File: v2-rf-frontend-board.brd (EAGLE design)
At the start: 86.6 x 43.9 mm, 150 parts, among them J1 1.27MM-SWD-CONNECTOR, J2 CON_SMA-ENDFIRE_EMERSON_EMERS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, J3 ROCKETNET-CONNECTOR-16M, J4 ZX62D-B-5P8, J5 BREAKOUT, J7 CON_HIROSE_DM3D(MICROSD), Q1 NTR4101P, T1 ALT4532, T2 ALT4532, U1 MAX2769, U2 STM32F4V_100PIN_GPSBOARD, U3 KSZ8081, U4 7Q-16.368MBG-T, U5 XC2401A8167R-G, U6 MAX8510EXK29+T, U7 MAX8510EXK29+T, U8 LMZ12001, X1 25 MHz

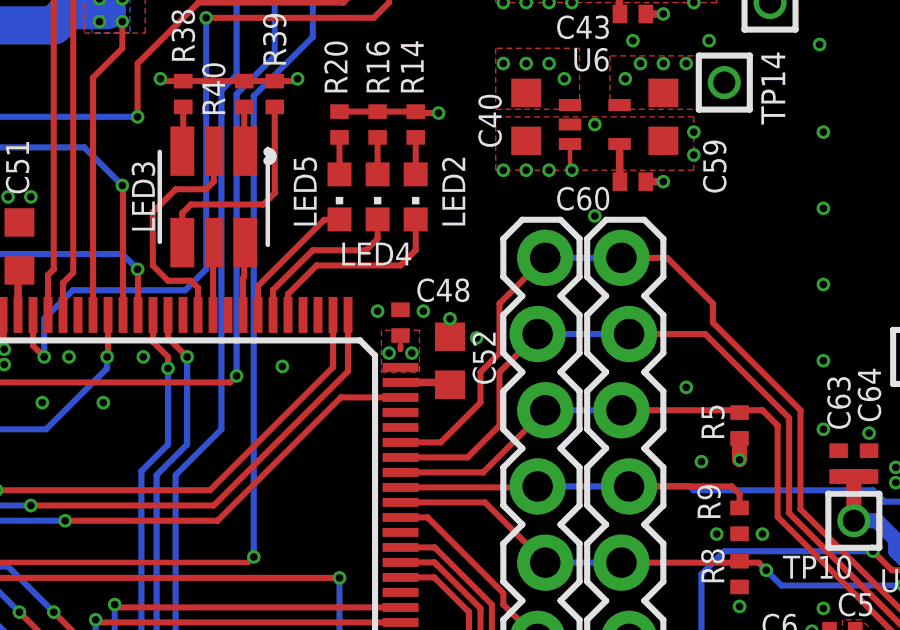
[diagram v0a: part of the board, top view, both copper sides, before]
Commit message: Silly clean up, ran ERC and DRC again.
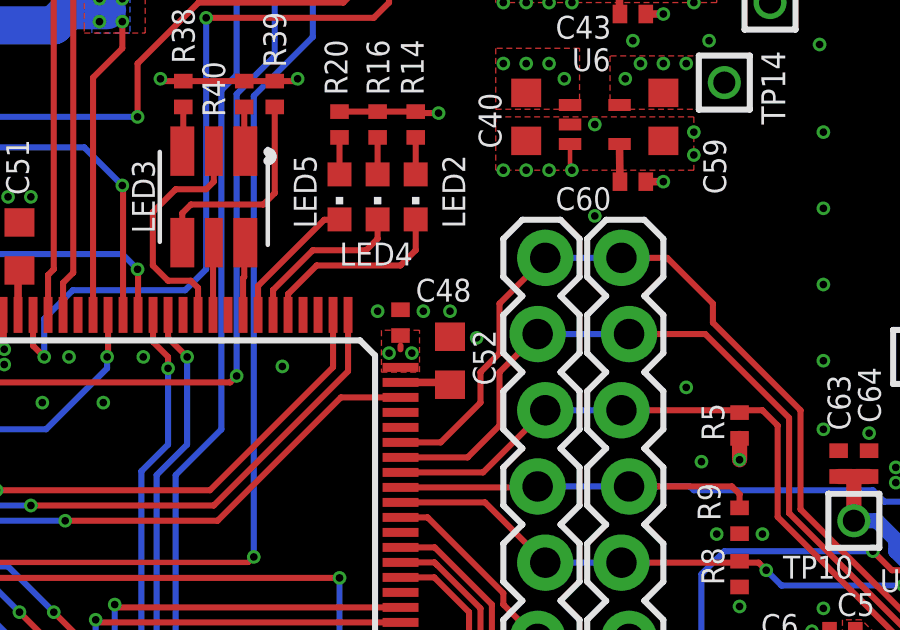
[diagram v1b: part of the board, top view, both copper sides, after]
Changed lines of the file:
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@@
 <layer number="23" name="tOrigins" color="15" fill="1" visible="yes" active="yes"/>
 <layer number="24" name="bOrigins" color="15" fill="1" visible="yes" active="yes"/>
-<layer number="25" name="tNames" color="7" fill="1" visible="yes" active="yes"/>
+<layer number="25" name="tNames" color="7" fill="1" visible="no" active="yes"/>
 <layer number="26" name="bNames" color="7" fill="1" visible="no" active="yes"/>
 <layer number="27" name="tValues" color="7" fill="1" visible="no" active="yes"/>
@@
 <via x="28.067" y="36.83" extent="1-16" drill="0.254"/>
 <via x="40.64" y="38.227" extent="1-16" drill="0.254"/>
-<via x="58.674" y="26.797" extent="1-16" drill="0.254"/>
+<via x="58.674" y="27.051" extent="1-16" drill="0.254"/>
 <via x="74.93" y="41.91" extent="1-16" drill="0.254"/>
 <via x="76.581" y="21.463" extent="1-16" drill="0.254"/>

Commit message: Added modwire proposals for SPI 3-wire fix. See Issue 4 in gps-rf-board github repository.
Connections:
- net MAX_CFG_!CS: now also U2.96
- net MAX_CFG_MOSI: now also U2.54
- net MAX_CFG_SCLK: now also U2.47
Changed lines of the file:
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@@
 <wire x1="69.977" y1="20.32" x2="69.977" y2="23.495" width="0.2032" layer="1"/>
 <wire x1="69.977" y1="23.495" x2="67.183" y2="26.289" width="0.2032" layer="1"/>
+<contactref element="U2" pad="47"/>
+<wire x1="57.026" y1="22.177" x2="57.026" y2="23.677" width="0" layer="19" extent="1-1"/>
 </signal>
 <signal name="MAX_CFG_MOSI">
@@
 <wire x1="70.358" y1="20.447" x2="70.358" y2="23.749" width="0.2032" layer="1"/>
 <wire x1="70.358" y1="23.749" x2="67.437" y2="26.67" width="0.2032" layer="1"/>
+<contactref element="U2" pad="54"/>
+<wire x1="57.026" y1="22.677" x2="53.776" y2="26.927" width="0" layer="19" extent="1-1"/>
 </signal>
 <signal name="MAX_CFG_!CS">
@@
 <wire x1="57.026" y1="21.677" x2="59.777" y2="21.677" width="0.2032" layer="1"/>
 <wire x1="59.777" y1="21.677" x2="61.849" y2="23.749" width="0.2032" layer="1"/>
+<contactref element="U2" pad="96"/>
+<wire x1="41.526" y1="15.177" x2="57.026" y2="21.677" width="0" layer="19" extent="1-1"/>
 </signal>
 <signal name="N$9">

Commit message: Removed SPI2_NSS modwire proposal from v2 schematic.
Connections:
- net MAX_CFG_!CS: no longer U2.96
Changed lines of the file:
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@@
 <wire x1="57.026" y1="21.677" x2="59.777" y2="21.677" width="0.2032" layer="1"/>
 <wire x1="59.777" y1="21.677" x2="61.849" y2="23.749" width="0.2032" layer="1"/>
-<contactref element="U2" pad="96"/>
-<wire x1="41.526" y1="15.177" x2="57.026" y2="21.677" width="0" layer="19" extent="1-1"/>
 </signal>
 <signal name="N$9">

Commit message: Added annotation for DEBUG-PHY-MODWIRE (currently on prototype)
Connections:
- removed net N$39: LED6.C, U3.23
- removed net N$57: TP1.1, U2.1
- new net DEBUG-PHY-MODWIRE: LED6.C, TP1.1, U2.1, U3.23
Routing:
- net DEBUG-PHY-MODWIRE: track 0.00 -> 10.4 mm, vias 0 -> 2
- net N$39: track 5.92 -> 0.00 mm, vias 2 -> 0
- net N$57: track 4.49 -> 0.00 mm
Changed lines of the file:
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@@
 <?xml version="1.0" encoding="utf-8"?>
 <!DOCTYPE eagle SYSTEM "eagle.dtd">
-<eagle version="6.6.0">
+<eagle version="6.5.0">
 <drawing>
 <settings>
@@
 </polygon>
 </signal>
-<signal name="N$39">
+<signal name="DEBUG-PHY-MODWIRE">
 <contactref element="U3" pad="23"/>
 <contactref element="LED6" pad="C"/>
@@
 <wire x1="26.936" y1="20.078" x2="26.936" y2="22.594" width="0.2286" layer="16"/>
 <wire x1="26.936" y1="22.594" x2="26.924" y2="22.606" width="0.2286" layer="16"/>
+<contactref element="TP1" pad="1"/>
+<contactref element="U2" pad="1"/>
+<wire x1="39.37" y1="10.795" x2="39.624" y2="10.795" width="0.2286" layer="1"/>
+<wire x1="39.624" y1="10.795" x2="40.64" y2="11.811" width="0.2286" layer="1"/>
+<wire x1="40.64" y1="11.811" x2="42.164" y2="11.811" width="0.2286" layer="1"/>
+<wire x1="42.164" y1="11.811" x2="42.545" y2="11.43" width="0.2286" layer="1"/>
+<wire x1="42.545" y1="11.43" x2="43.273" y2="11.43" width="0.2286" layer="1"/>
+<wire x1="43.273" y1="11.43" x2="43.276" y2="11.427" width="0.2286" layer="1"/>
+<wire x1="26.936" y1="17.862" x2="39.37" y2="10.795" width="0" layer="19" extent="1-1"/>
 </signal>
 <signal name="N$24">
@@
 <wire x1="42.164" y1="10.795" x2="41.148" y2="10.795" width="0.2286" layer="1"/>
 </signal>
-<signal name="N$57">
-<contactref element="TP1" pad="1"/>
-<contactref element="U2" pad="1"/>
-<wire x1="39.37" y1="10.795" x2="39.624" y2="10.795" width="0.2286" layer="1"/>
-<wire x1="39.624" y1="10.795" x2="40.64" y2="11.811" width="0.2286" layer="1"/>
-<wire x1="40.64" y1="11.811" x2="42.164" y2="11.811" width="0.2286" layer="1"/>
-<wire x1="42.164" y1="11.811" x2="42.545" y2="11.43" width="0.2286" layer="1"/>
-<wire x1="42.545" y1="11.43" x2="43.273" y2="11.43" width="0.2286" layer="1"/>
-<wire x1="43.273" y1="11.43" x2="43.276" y2="11.427" width="0.2286" layer="1"/>
-</signal>
 <signal name="USART6_TX">

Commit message: Added modwire for SPI1-NSS. This should enable the use of STM32 SPI1 in slave mode to read data output.
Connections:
- new net N$3: U2.35
- new net SPI1-NSS: U2.29, U2.31
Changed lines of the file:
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@@
 <wire x1="31.623" y1="10.668" x2="33.02" y2="10.668" width="0.2032" layer="16"/>
+</signal>
+<signal name="N$3">
+<contactref element="U2" pad="35"/>
+</signal>
+<signal name="SPI1-NSS">
+<contactref element="U2" pad="29"/>
+<contactref element="U2" pad="31"/>
+<wire x1="57.026" y1="14.677" x2="57.026" y2="15.677" width="0" layer="19" extent="1-1"/>
 </signal>
 </signals>
